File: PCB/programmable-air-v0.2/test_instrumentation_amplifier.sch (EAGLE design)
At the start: 15 parts, among them IC1 INA126U, IC2 7805T

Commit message: Working towards instrumentation amplifier instead of HX711
MCP6001 was a huge mistake. 6V Vin max. Modifying circuit to LM358.
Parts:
- R4, R5, R6, R7: device eagle-ltspice:RR0603 -> eagle-ltspice:R0207/10
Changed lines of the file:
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@@
 <?xml version="1.0" encoding="utf-8"?>
 <!DOCTYPE eagle SYSTEM "eagle.dtd">
-<eagle version="8.7.0">
+<eagle version="9.0.1">
 <drawing>
 <settings>
@@
 <layer number="18" name="Vias" color="2" fill="1" visible="no" active="no"/>
 <layer number="19" name="Unrouted" color="6" fill="1" visible="no" active="no"/>
-<layer number="20" name="Dimension" color="15" fill="1" visible="no" active="no"/>
+<layer number="20" name="Dimension" color="24" fill="1" visible="no" active="no"/>
 <layer number="21" name="tPlace" color="7" fill="1" visible="no" active="no"/>
 <layer number="22" name="bPlace" color="7" fill="1" visible="no" active="no"/>
@@
 <part name="R2" library="eagle-ltspice" library_urn="urn:adsk.eagle:library:217" deviceset="R" device="R0603" package3d_urn="urn:adsk.eagle:package:13302/1" value="10K"/>
 <part name="R3" library="eagle-ltspice" library_urn="urn:adsk.eagle:library:217" deviceset="R" device="R0603" package3d_urn="urn:adsk.eagle:package:13302/1" value="20K"/>
-<part name="R4" library="eagle-ltspice" library_urn="urn:adsk.eagle:library:217" deviceset="R" device="R0603" package3d_urn="urn:adsk.eagle:package:13302/1" value="20K"/>
-<part name="R5" library="eagle-ltspice" library_urn="urn:adsk.eagle:library:217" deviceset="R" device="R0603" package3d_urn="urn:adsk.eagle:package:13302/1" value="20K"/>
-<part name="R6" library="eagle-ltspice" library_urn="urn:adsk.eagle:library:217" deviceset="R" device="R0603" package3d_urn="urn:adsk.eagle:package:13302/1" value="19.9K"/>
-<part name="R7" library="eagle-ltspice" library_urn="urn:adsk.eagle:library:217" deviceset="R" device="R0603" package3d_urn="urn:adsk.eagle:package:13302/1" value="20K"/>
+<part name="R4" library="eagle-ltspice" library_urn="urn:adsk.eagle:library:217" deviceset="R" device="0207/10" package3d_urn="urn:adsk.eagle:package:13275/1" value="20K"/>
+<part name="R5" library="eagle-ltspice" library_urn="urn:adsk.eagle:library:217" deviceset="R" device="0207/10" package3d_urn="urn:adsk.eagle:package:13275/1" value="20K"/>
+<part name="R6" library="eagle-ltspice" library_urn="urn:adsk.eagle:library:217" deviceset="R" device="0207/10" package3d_urn="urn:adsk.eagle:package:13275/1" value="19.9K"/>
+<part name="R7" library="eagle-ltspice" library_urn="urn:adsk.eagle:library:217" deviceset="R" device="0207/10" package3d_urn="urn:adsk.eagle:package:13275/1" value="20K"/>
 <part name="R8" library="eagle-ltspice" library_urn="urn:adsk.eagle:library:217" deviceset="R" device="R0603" package3d_urn="urn:adsk.eagle:package:13302/1" value="1.78K"/>
 <part name="R9" library="eagle-ltspice" library_urn="urn:adsk.eagle:library:217" deviceset="R" device="R0603" package3d_urn="urn:adsk.eagle:package:13302/1" value="2K"/>

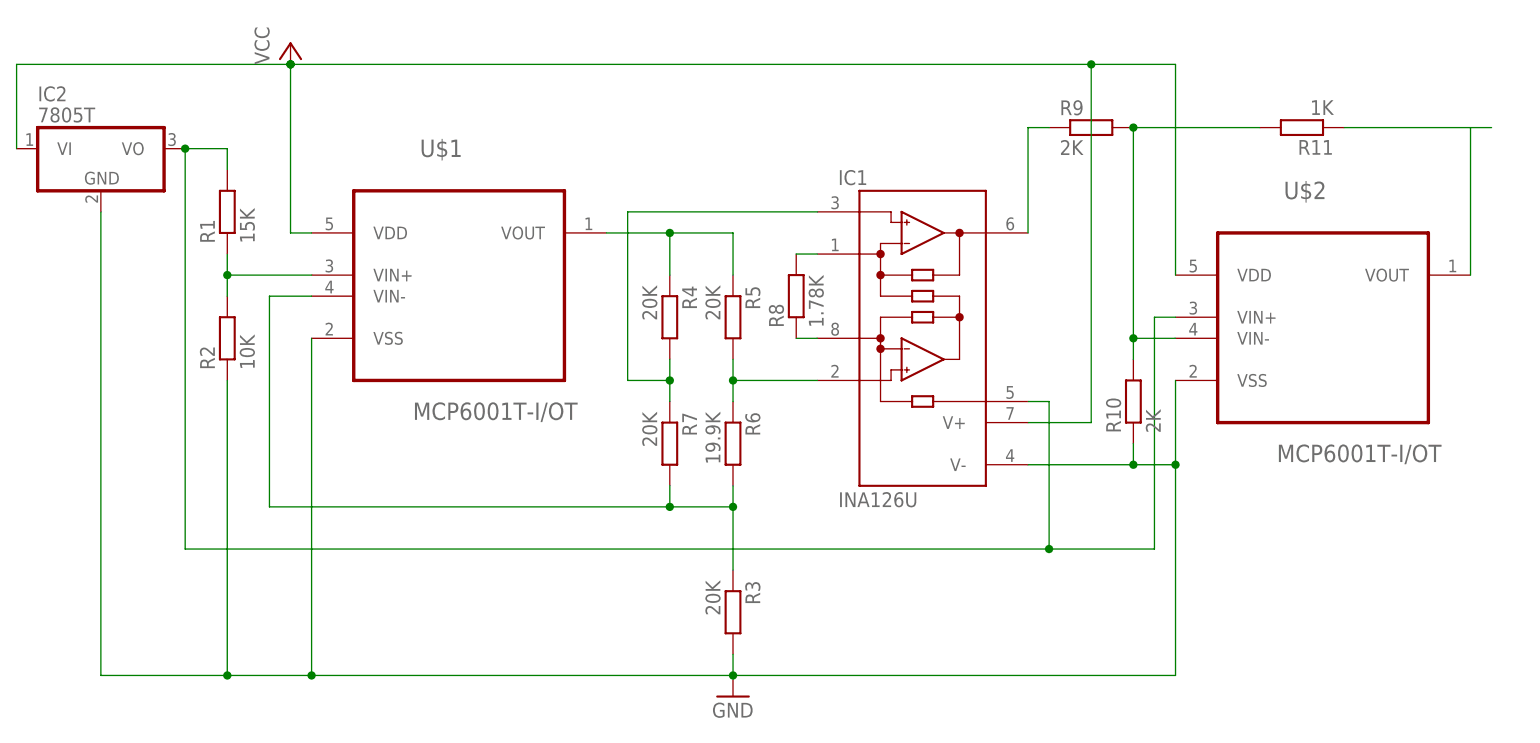
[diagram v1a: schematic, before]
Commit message: LM358 test board ready
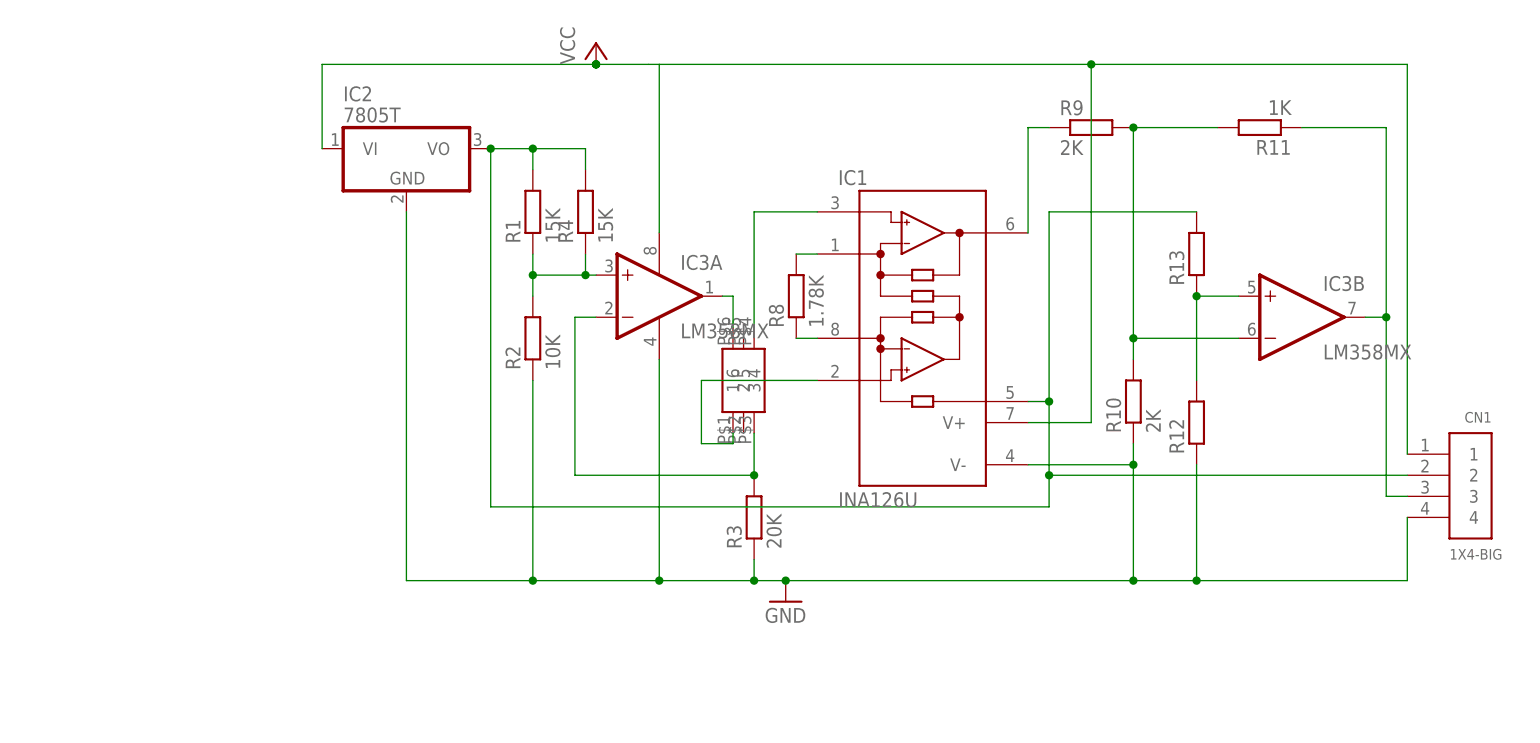
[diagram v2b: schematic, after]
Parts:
- removed R5, R7: 20K, eagle-ltspice:R0207/10
- removed R6: 19.9K, eagle-ltspice:R0207/10
- removed U$2: MCP6001T-I/OT, MCP6001T-I_OT:MCP6001T-I/OT
- added CN1: 1X4-BIG, adafruit:1X4-BIG
- added IC3: LM358MX, linear:LM358MX
- added R12, R13: (no value), eagle-ltspice:R0207/10
- R1, R10, R11, R2, R3, R8, R9: device eagle-ltspice:RR0603 -> eagle-ltspice:R0207/10
- R4: value 20K -> 15K
- U$1: value MCP6001T-I/OT -> 2SMPP-03; device MCP6001T-I_OT:MCP6001T-I/OT -> programmable-air-components:2SMPP-03; SPICEPREFIX X -> (none)
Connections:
- removed net N$6: R3.1, R6.2, R7.2, U$1.VIN-
- new net N$11: IC3B.+IN, R12.2, R13.1
- new net N$13: IC3A.-IN, R3.2, U$1.3
- net GND: now also CN1.4, IC3P.V-, R12.1, R3.1; no longer R3.2, U$1.VSS, U$2.VSS
- net N$1: now also IC3B.-IN; no longer U$2.VIN-
- net N$10: now also IC3A.+IN, R4.1; no longer U$1.VIN+
- net N$12: now also CN1.3, IC3B.OUT; no longer U$2.VOUT
- net N$3: now also U$1.4; no longer R4.2, R7.1
- net N$4: now also CN1.2, R13.2, R4.2; no longer U$2.VIN+
- net N$7: now also U$1.1; no longer R5.2, R6.1
- net N$8: now also IC3A.OUT, U$1.6; no longer R4.1, R5.1, U$1.VOUT
- net VCC: now also CN1.1, IC3P.V+; no longer U$1.VDD, U$2.VDD
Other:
- moved on the sheet: IC2, R1, R11, R2, R3, R4
